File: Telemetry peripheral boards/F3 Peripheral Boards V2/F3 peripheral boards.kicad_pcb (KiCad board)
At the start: 2 copper layers, 52 parts, among them J1 ATS668LSM, J2 Conn_01x04_MountingPin, J3 Potentiometer, J4 Strain Gauge, J5 Tire temp Sensor, U1 LM2907M/NOPB, U2 INA125U, U3 MCP2515-I/SO, U4 ISO1050DUB, U5 ATtiny1616-S, U6 LM7805CV, U7 LF33CV, Y1 Crystal

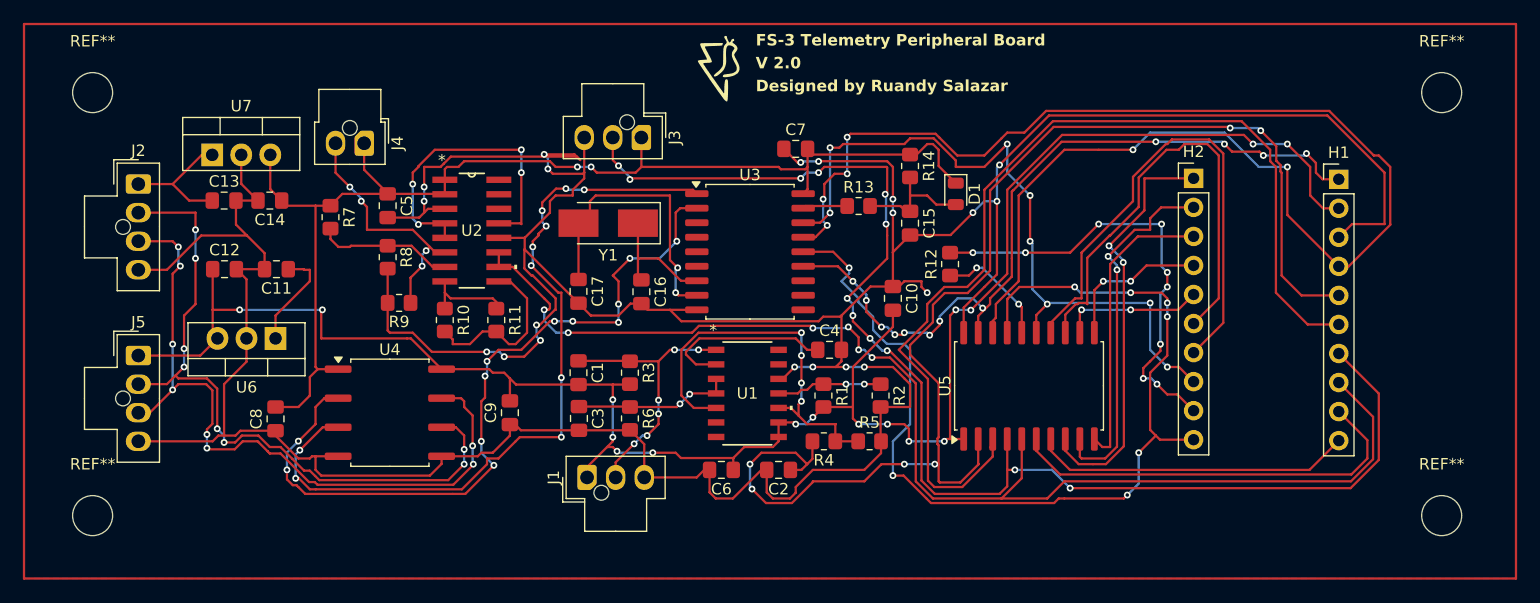
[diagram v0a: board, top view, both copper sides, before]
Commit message: Edge cuts and mounting holes updated
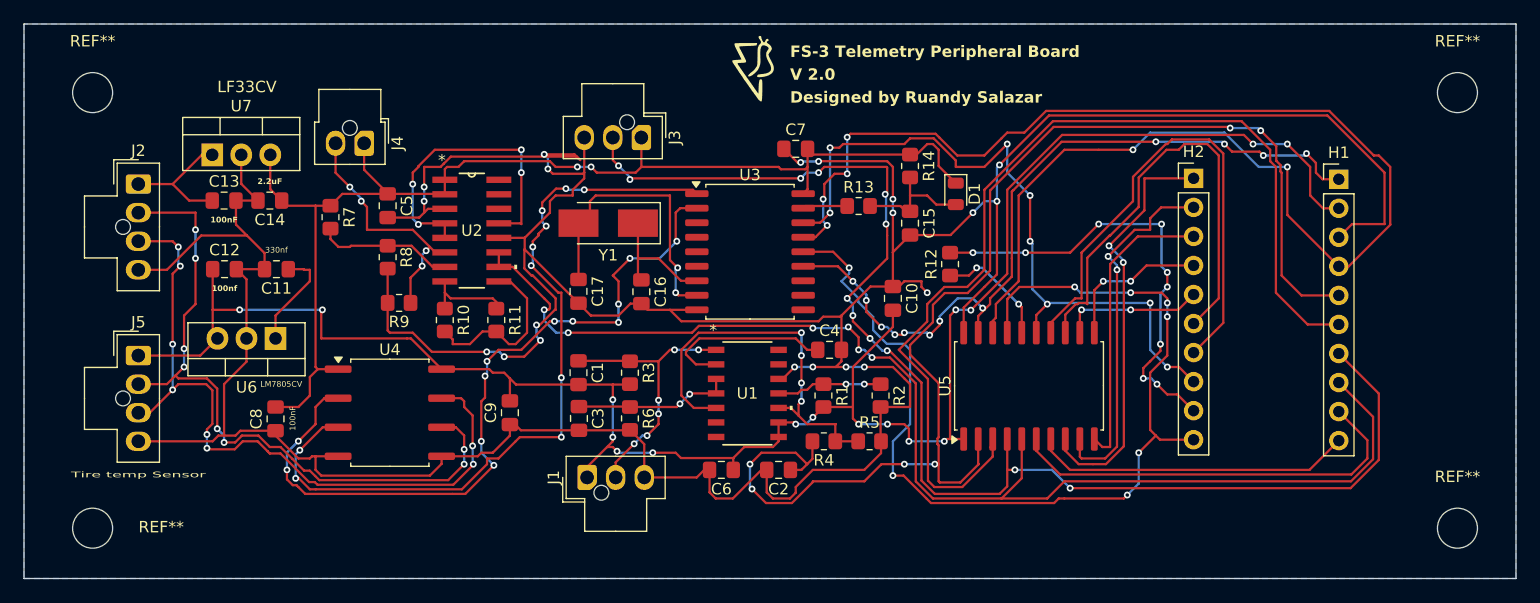
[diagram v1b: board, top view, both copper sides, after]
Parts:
- moved G*** 3.00 mm to (121.5, 35.5)
- moved REF** 1.76 mm to (182.9, 75.6)
- moved REF** 1.38 mm to (182.9, 37.5)
- moved REF** 1.10 mm to (63.5, 75.6)
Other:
- board outline added: 130.5 x 48.5 mm
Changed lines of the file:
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@@
 		(tags "Through hole pin header THT 1x10 2.54mm single row")
 		(property "Reference" "H2"
-			(at 0 -2.33 360)
+			(at 0 -2.33 0)
 			(layer "F.SilkS")
 			(effects
@@
 		)
 		(property "Value" "Conn_01x10_MountingPin"
-			(at 0 25.19 360)
+			(at 0 25.19 0)
 			(layer "F.Fab")
 			(effects
@@
 		(tags "TO-220-3 Vertical RM 2.54mm")
 		(property "Reference" "U6"
-			(at 2.54 -4.27 360)
+			(at 2.54 -4.27 0)
 			(layer "F.SilkS")
 			(effects
@@
 		)
 		(property "Value" "LM7805CV"
-			(at 2.54 2.5 360)
-			(layer "F.Fab")
+			(at -0.5 -4 0)
+			(layer "F.SilkS")
 			(effects
 				(font
-					(size 1 1)
-					(thickness 0.15)
+					(size 0.5 0.5)
+					(thickness 0.1)
 				)
 			)
 		)
 		(property "Footprint" "Package_TO_SOT_THT:TO-220-3_Vertical"
-			(at 0 0 360)
+			(at 0 0 0)
 			(layer "F.Fab")
 			(hide yes)
@@
 		)
 		(property "Datasheet" "https://www.onsemi.cn/PowerSolutions/document/MC7800-D.PDF"
-			(at 0 0 360)
+			(at 0 0 0)
 			(layer "F.Fab")
 			(hide yes)
@@
 		)
 		(property "Description" ""
-			(at 0 0 360)
+			(at 0 0 0)
 			(layer "F.Fab")
 			(hide yes)
@@
 		)
 		(fp_text user "${REFERENCE}"
-			(at 2.54 -4.27 360)
+			(at 2.54 -4.27 0)
 			(layer "F.Fab")
 			(effects
@@
 	(footprint "1FS_2_Global_Footprint_Library:FS_Logo_4LinesTall"
 		(layer "F.Cu")
-		(at 118.5 35.5)
+		(at 121.5 35.5)
 		(property "Reference" "G***"
 			(at 0 0 0)
@@
 		(tags "Through hole pin header THT 1x10 2.54mm single row")
 		(property "Reference" "H1"
-			(at 0 -2.33 360)
+			(at 0 -2.33 0)
 			(layer "F.SilkS")
 			(effects
@@
 		)
 		(property "Value" "Conn_01x10_MountingPin"
-			(at 0 25.19 360)
+			(at 0 25.19 0)
 			(layer "F.Fab")
 			(effects
@@
 		)
 		(property "Value" "LF33CV"
-			(at 2.54 2.5 0)
-			(layer "F.Fab")
+			(at 3.04 -5.945 0)
+			(layer "F.SilkS")
 			(effects
 				(font
@@
 		(tags "capacitor handsolder")
 		(property "Reference" "C2"
-			(at 0 -1.68 360)
+			(at 0 -1.68 0)
 			(layer "F.SilkS")
 			(effects
@@
 		)
 		(property "Value" "100nF"
-			(at 0 1.68 360)
+			(at 0 1.68 0)
 			(layer "F.Fab")
 			(effects
@@
 		)
 		(fp_text user "${REFERENCE}"
-			(at 0 0 360)
+			(at 0 0 0)
 			(layer "F.Fab")
 			(effects
@@
 	(footprint "MountingHole:MountingHole_3.5mm"
 		(layer "F.Cu")
-		(at 181.5 37.5)
+		(at 182.88 37.5)
 		(descr "Mounting Hole 3.5mm, no annular")
 		(tags "mounting hole 3.5mm no annular")
@@
 		(tags "capacitor handsolder")
 		(property "Reference" "C6"
-			(at 0 -1.68 360)
+			(at 0 -1.68 0)
 			(layer "F.SilkS")
 			(effects
@@
 		)
 		(property "Value" "100nF"
-			(at 0 1.68 360)
+			(at 0 1.68 0)
 			(layer "F.Fab")
 			(effects
@@
 		)
 		(fp_text user "${REFERENCE}"
-			(at 0 0 360)
+			(at 0 0 0)
 			(layer "F.Fab")
 			(effects
@@
 		)
 		(property "Value" "100nF"
-			(at 0 1.68 90)
-			(layer "F.Fab")
+			(at 0.0375 1.5 90)
+			(layer "F.SilkS")
 			(effects
 				(font
-					(size 1 1)
-					(thickness 0.15)
+					(size 0.5 0.5)
+					(thickness 0.1)
 				)
 			)
@@
 		(tags "capacitor handsolder")
 		(property "Reference" "C14"
-			(at 0 -1.68 360)
+			(at 0 -1.68 0)
 			(layer "F.SilkS")
 			(effects
@@
 		)
 		(property "Value" "2.2uF"
-			(at 0 1.68 360)
-			(layer "F.Fab")
+			(at 0 1.68 0)
+			(layer "F.SilkS")
 			(effects
 				(font
-					(size 1 1)
-					(thickness 0.15)
+					(size 0.5 0.5)
+					(thickness 0.1)
+					(bold yes)
 				)
 			)
@@
 		)
 		(fp_text user "${REFERENCE}"
-			(at 0 0 360)
+			(at 0 0 0)
 			(layer "F.Fab")
 			(effects
@@
 	(footprint "MountingHole:MountingHole_3.5mm"
 		(layer "F.Cu")
-		(at 181.5 74.5)
+		(at 182.88 75.6)
 		(descr "Mounting Hole 3.5mm, no annular")
 		(tags "mounting hole 3.5mm no annular")
@@
 		(tags "resistor handsolder")
 		(property "Reference" "R4"
-			(at 0 -1.65 360)
+			(at 0 -1.65 0)
 			(layer "F.SilkS")
 			(effects
@@
 		)
 		(property "Value" "100K"
-			(at 0 1.65 360)
+			(at 0 1.65 0)
 			(layer "F.Fab")
 			(effects
@@
 		)
 		(fp_text user "${REFERENCE}"
-			(at 0 0 360)
+			(at 0 0 0)
 			(layer "F.Fab")
 			(effects
@@
 		(tags "capacitor handsolder")
 		(property "Reference" "C12"
-			(at 0 -1.68 360)
+			(at 0 -1.68 0)
 			(layer "F.SilkS")
 			(effects
@@
 		)
 		(property "Value" "100nf"
-			(at 0 1.68 360)
-			(layer "F.Fab")
+			(at 0 1.68 0)
+			(layer "F.SilkS")
 			(effects
 				(font
-					(size 1 1)
-					(thickness 0.15)
+					(size 0.5 0.5)
+					(thickness 0.1)
+					(bold yes)
 				)
 			)
@@
 		)
 		(fp_text user "${REFERENCE}"
-			(at 0 0 360)
+			(at 0 0 0)
 			(layer "F.Fab")
 			(effects
@@
 		(tags "resistor handsolder")
 		(property "Reference" "R9"
-			(at 0 -1.65 360)
+			(at 0 -1.65 0)
 			(layer "F.SilkS")
 			(effects
@@
 		)
 		(property "Value" "120"
-			(at 0 1.65 360)
+			(at 0 1.65 0)
 			(layer "F.Fab")
 			(effects
@@
 		)
 		(fp_text user "${REFERENCE}"
-			(at 0 0 360)
+			(at 0 0 0)
 			(layer "F.Fab")
 			(effects
@@
 		(property "Value" "Tire temp Sensor"
 			(at 0 10.42 0)
-			(layer "F.Fab")
+			(layer "F.SilkS")
 			(effects
 				(font
-					(size 1 1)
-					(thickness 0.15)
+					(size 0.5 1)
+					(thickness 0.1)
 				)
 			)
@@
 		(tags "connector Molex Nano-Fit side entry")
 		(property "Reference" "J2"
-			(at 0 -2.92 360)
+			(at 0 -2.92 0)
 			(layer "F.SilkS")
 			(effects
@@
 		)
 		(property "Value" "Conn_01x04_MountingPin"
-			(at 0 10.42 360)
+			(at 0 10.42 0)
 			(layer "F.Fab")
 			(effects
@@
 		)
 		(property "Footprint" "Molex Nanofit:Molex_Nano-Fit_105309-xx04_1x04_P2.50mm_Vertical"
-			(at 0 0 360)
+			(at 0 0 0)
 			(layer "F.Fab")
 			(hide yes)
@@
 		)
 		(property "Datasheet" ""
-			(at 0 0 360)
+			(at 0 0 0)
 			(layer "F.Fab")
 			(hide yes)
@@
 		)
 		(property "Description" "Generic connectable mounting pin connector, single row, 01x04, script generated (kicad-library-utils/schlib/autogen/connector/)"
-			(at 0 0 360)
+			(at 0 0 0)
 			(layer "F.Fab")
 			(hide yes)
@@
 		(property "Value" "100nF"
 			(at 0 1.68 0)
-			(layer "F.Fab")
+			(layer "F.SilkS")
 			(effects
 				(font
-					(size 1 1)
-					(thickness 0.15)
+					(size 0.5 0.5)
+					(thickness 0.1)
+					(bold yes)
 				)
 			)
@@
 		)
 		(fp_text user "${REFERENCE}"
-			(at 1.1 2.5 360)
+			(at 1.1 2.5 0)
 			(layer "F.Fab")
 			(effects
@@
 		(tags "SMD SMT crystal hand-soldering")
 		(property "Reference" "Y1"
-			(at 0 -2.8 360)
+			(at 0 -2.8 0)
 			(layer "F.SilkS")
 			(effects
@@
 		)
 		(property "Value" "Crystal"
-			(at 0 2.8 360)
+			(at 0 2.8 0)
 			(layer "F.Fab")
 			(effects
@@
 		)
 		(fp_text user "${REFERENCE}"
-			(at 0 0 360)
+			(at 0 0 0)
 			(layer "F.Fab")
 			(effects
@@
 		(tags "capacitor handsolder")
 		(property "Reference" "C11"
-			(at 0 -1.68 360)
+			(at 0 -1.68 0)
 			(layer "F.SilkS")
 			(effects
@@
 		)
 		(property "Value" "330nf"
-			(at 0 1.68 360)
-			(layer "F.Fab")
+			(at 0 1.68 0)
+			(layer "F.SilkS")
 			(effects
 				(font
-					(size 1 1)
-					(thickness 0.15)
+					(size 0.5 0.5)
+					(thickness 0.1)
 				)
 			)
@@
 		)
 		(fp_text user "${REFERENCE}"
-			(at 0 0 360)
+			(at 0 0 0)
 			(layer "F.Fab")
 			(effects
@@
 		)
 		(fp_text user "${REFERENCE}"
-			(at 1.1 2.5 360)
+			(at 1.1 2.5 0)
 			(layer "F.Fab")
 			(effects
@@
 	(footprint "MountingHole:MountingHole_3.5mm"
 		(layer "F.Cu")
-		(at 63.5 74.5)
+		(at 63.5 75.6)
 		(descr "Mounting Hole 3.5mm, no annular")
 		(tags "mounting hole 3.5mm no annular")
 		(property "Reference" "REF**"
-			(at 0 -4.5 0)
+			(at 6 -0.1 0)
 			(layer "F.SilkS")
 			(effects
@@
 		(end 188 80)
 		(stroke
-			(width 0.2)
+			(width 0.05)
 			(type default)
 		)
 		(fill none)
-		(layer "F.Cu")
+		(layer "Edge.Cuts")
 	)
 	(gr_text "V 2.0"
-		(at 121.5 35.5 0)
+		(at 124.5 36.5 0)
 		(layer "F.SilkS")
 		(effects
@@
 	)
 	(gr_text "FS-3 Telemetry Peripheral Board"
-		(at 121.5 33.5 0)
+		(at 124.5 34.5 0)
 		(layer "F.SilkS")
 		(effects
@@
 	)
 	(gr_text "Designed by Ruandy Salazar"
-		(at 121.5 37.5 0)
+		(at 124.5 38.5 0)
 		(layer "F.SilkS")
 		(effects
